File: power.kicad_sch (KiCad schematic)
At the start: 32 parts, among them J4 USB_C_Receptacle_USB2.0_16P, J7 Ext VCC Out, SW2 Slide_DPDT_SS22D06, U2 TPS7A0333PDBVR, U3 MCP73831T-2ACI/OT

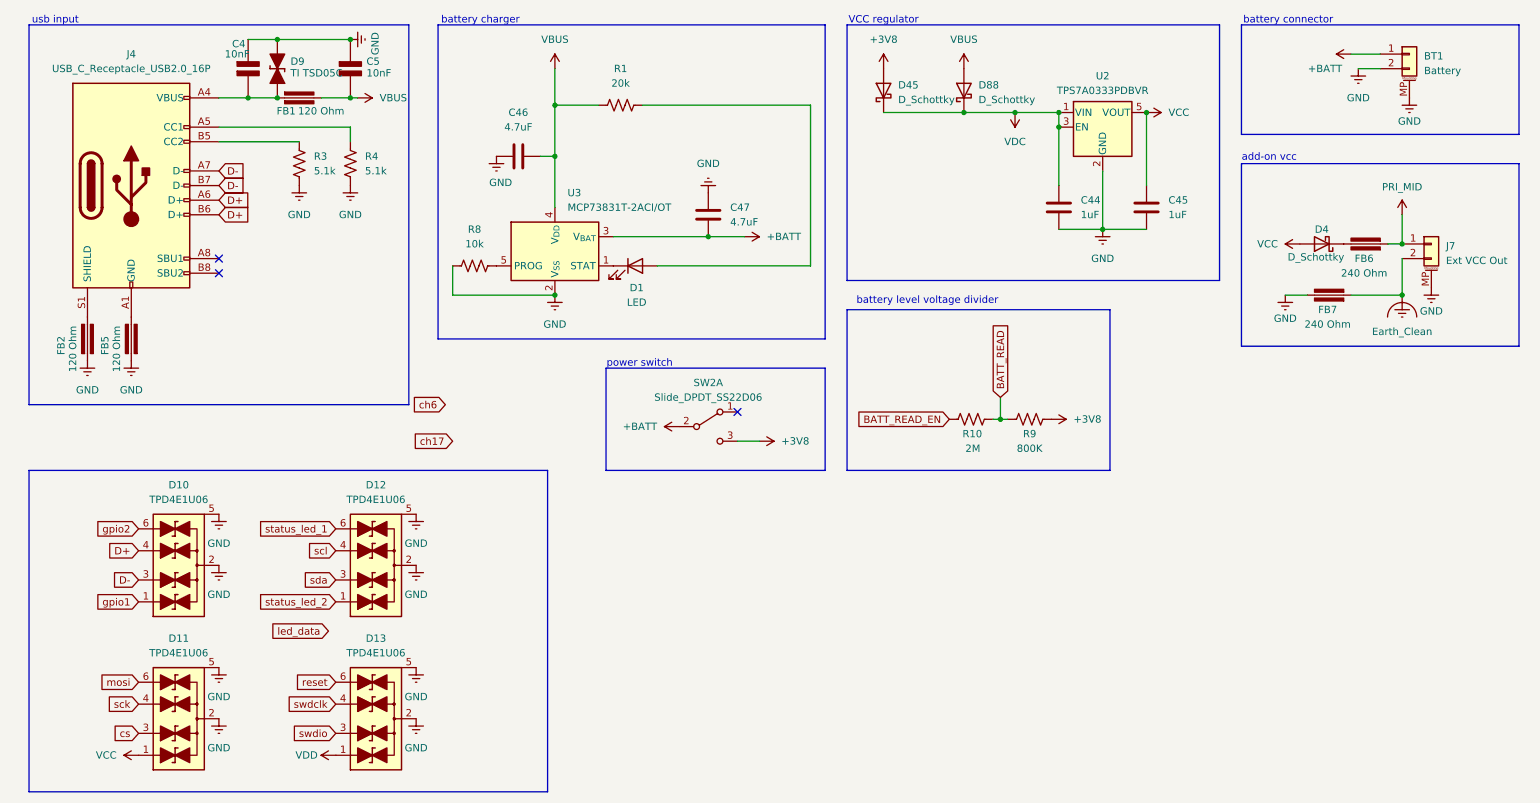
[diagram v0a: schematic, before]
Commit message: mariposa v2 RC3
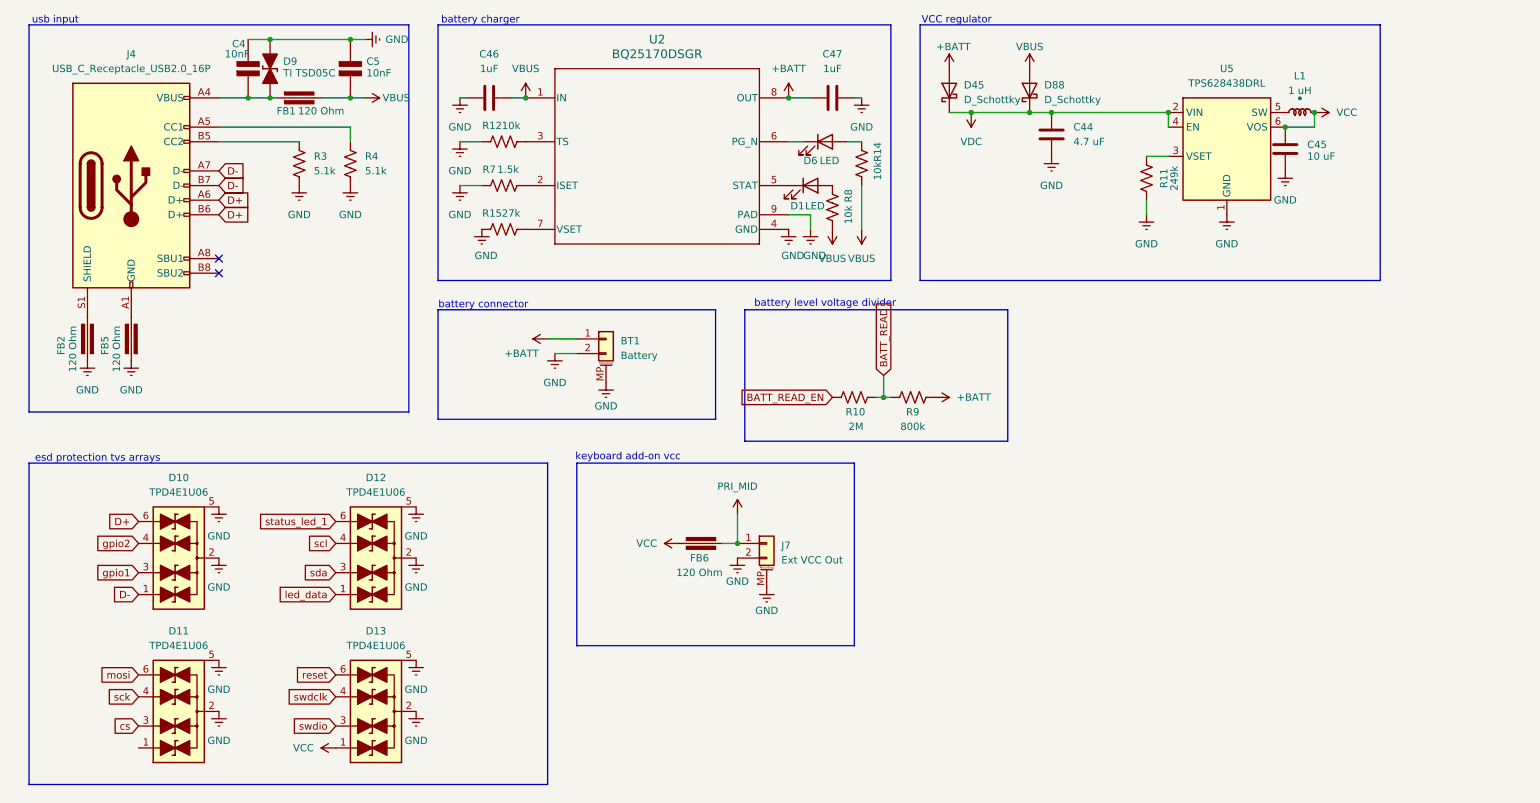
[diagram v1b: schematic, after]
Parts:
- removed D4: D_Schottky, PCM_Diode_SMD_Handsoldering_AKL:D_SOD-123F, symbol Device:D_Schottky
- removed FB7: 240 Ohm, PCM_Ferrite_SMD_AKL:Ferrite_0603_1608Metric, symbol PCM_Device_AKL:Ferrite_Bead
- removed R1: 20k, Resistor_SMD:R_0603_1608Metric, symbol Device:R_US
- removed SW2: Slide_DPDT_SS22D06, Button_Switch_SMD:SW_DPDT_CK_JS202011JCQN, symbol PCM_4ms_Switch:Slide_DPDT_SS22D06
- removed U2: TPS7A0333PDBVR, Package_TO_SOT_SMD:SOT-23-5, symbol Regulator_Linear:AP2112K-3.3
- removed U3: MCP73831T-2ACI/OT, Package_TO_SOT_SMD:SOT-23-5, symbol Battery_Management:MCP73831-2-OT
- added D6: LED, coquette_footprints:LED 1206 reverse mount rectangle, symbol Device:LED
- added L1: 1 uH, Inductor_SMD:L_0603_1608Metric, symbol PCM_Generic-50:L,IEEE
- added R11: 249k, Resistor_SMD:R_0603_1608Metric, symbol Device:R_US
- added R12, R14: 10k, Resistor_SMD:R_0603_1608Metric, symbol Device:R_US
- added R15: 27k, Resistor_SMD:R_0603_1608Metric, symbol Device:R_US
- added R7: 1.5k, Resistor_SMD:R_0603_1608Metric, symbol Device:R_US
- added U2: BQ25170DSGR, coquette_footprints:DSG0008A, symbol coquette_symbols:BQ25170DSGR
- added U5: TPS628438DRL, Package_TO_SOT_SMD:SOT-563, symbol Regulator_Switching:TPS628438DRL
- C4, C5: footprint Capacitor_SMD:C_0402_1005Metric -> Capacitor_SMD:C_0603_1608Metric
- C44: value 1uF -> 4.7 uF
- C45: value 1uF -> 10 uF
- C46, C47: value 4.7uF -> 1uF
- D1: footprint PCM_LED_SMD_AKL:LED_1206_3216Metric_ReverseMount_Hole1.8x2.4mm -> coquette_footprints:LED 1206 reverse mount rectangle
- FB6: value 240 Ohm -> 120 Ohm
- R9: value 800K -> 800k
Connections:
- net +3V8 is gone; now on net +BATT: D45.2 (A), R9.1
- net Earth_Clean is gone; now on net GND: J7.2 (Pin_2)
- net VDD is gone; now on net VCC: D13.1 (L1)
- net status_led_2 is gone; now on net led_data: D12.1 (L1)
- net +BATT: now also U2.8 (OUT)
- net D+: now also D10.6 (L4); no longer D10.4 (L3)
- net D-: now also D10.1 (L1); no longer D10.3 (L2)
- net GND: now also R11.2, R12.2, R15.2, R7.2, U2.4 (GND), U2.9 (PAD), U5.1 (GND); no longer R8.2
- net VBUS: now also R8.1, R14.1, U2.1 (IN)
- net VCC: now also FB6.2, L1.2 (-), U5.6 (VOS); no longer D11.1 (L1)
- net VDC: now also U5.2 (VIN), U5.4 (EN)
- net gpio1: now also D10.3 (L2); no longer D10.1 (L1)
- net gpio2: now also D10.4 (L3); no longer D10.6 (L4)
- net at D1.1 (K): now also U2.5 (STAT)
- net at D1.2 (A): now also R8.2
- new net: R7.1, U2.2 (ISET)
- new net: R11.1, U5.3 (VSET)
- new net: L1.1 (+), U5.5 (SW)
- new net: R12.1, U2.3 (TS)
- new net: D6.1 (K), U2.6 (PG_N)
- new net: R15.1, U2.7 (VSET)
- new net: D6.2 (A), R14.2
- no-connect marks 3 -> 2
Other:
- note added: "esd protection tvs arrays"
- note added: "keyboard add-on vcc"
- note removed: "add-on vcc"
- note removed: "power switch"
- moved on the sheet: BT1, C44, C45, C46, C47, D1, D10, D11, D12, D13, D45, D88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
